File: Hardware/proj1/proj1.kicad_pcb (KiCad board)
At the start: 2 copper layers, 0 parts

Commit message: LED project layout
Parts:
- added D1: Red, layout:LED_0603_Symbol_on_F.SilkS, F.Cu at (119.5, 111.0)
- added J1: Conn_01x02, Connector_Molex:Molex_KK-254_AE-6410-02A_1x02_P2.54mm_Vertical, F.Cu at (103.0, 115.5)
- added R1: 105, Resistor_SMD:R_0603_1608Metric_Pad0.98x0.95mm_HandSolder, F.Cu at (119.6, 107.0)
- added SW1: SW_Push, Button_Switch_THT:SW_PUSH_6mm, F.Cu at (109.2, 107.8)
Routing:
- net +3V3: track 0.00 -> 21.1 mm
- net GND: track 0.00 -> 16.7 mm
- net Net-(D1-A): track 0.00 -> 9.97 mm
- net Net-(R1-Pad1): track 0.00 -> 9.74 mm
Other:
- board outline added: 25 x 20 mm

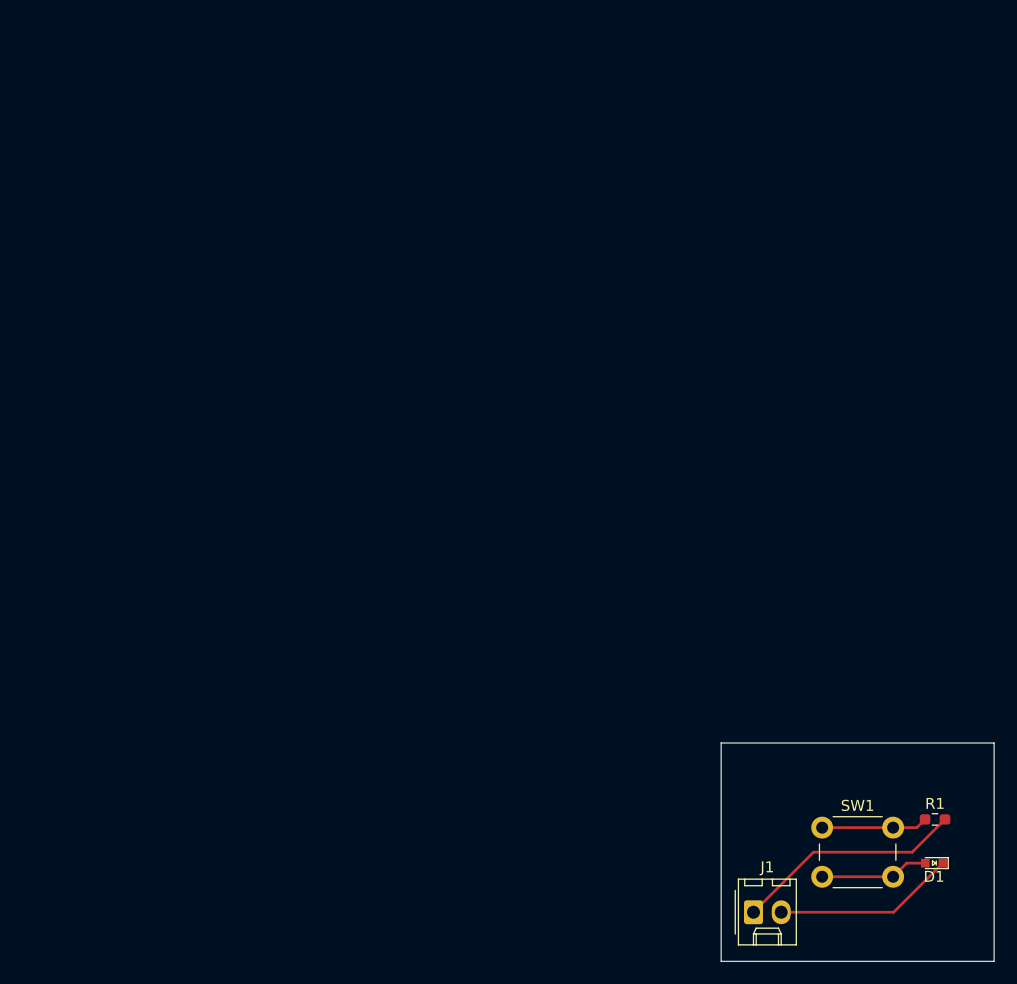
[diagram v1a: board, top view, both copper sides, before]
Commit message: Redo LED board PCB
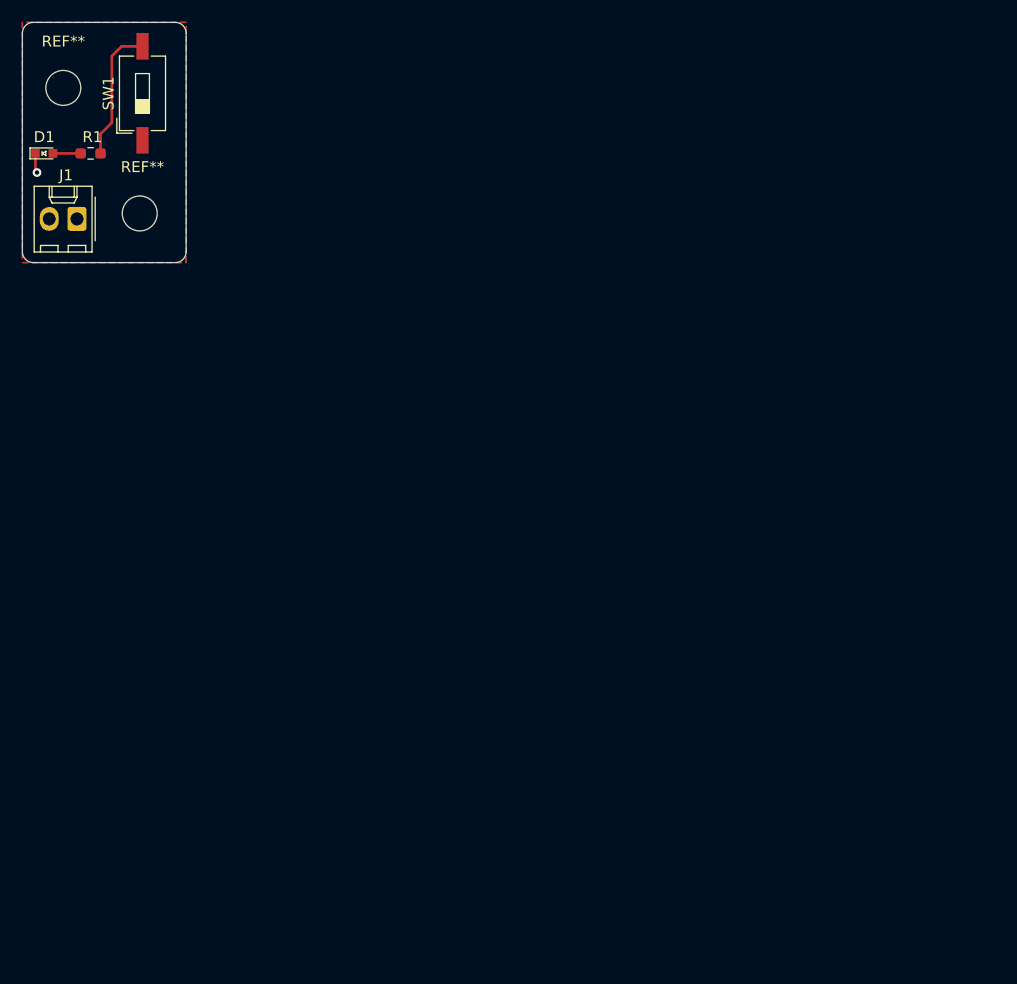
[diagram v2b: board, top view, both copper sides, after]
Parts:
- added REF**: MountingHole_3.2mm_M3, MountingHole:MountingHole_3.2mm_M3, F.Cu at (39.8, 40.0)
- added REF**: MountingHole_3.2mm_M3, MountingHole:MountingHole_3.2mm_M3, F.Cu at (46.8, 51.5)
- SW1: footprint Button_Switch_THT:SW_PUSH_6mm -> Button_Switch_SMD:SW_DIP_SPSTx01_Slide_6.7x4.1mm_W8.61mm_P2.54mm_LowProfile
- moved D1 104.2 mm to (38.0, 46.0), turned to 0 degrees
- moved R1 98.5 mm to (42.2, 46.0), turned to 180 degrees
- moved SW1 91.6 mm to (47.0, 40.5), turned to 90 degrees
- moved J1 88.7 mm to (41.0, 52.0), turned to 180 degrees
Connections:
- J1 pad 1: +3V3 -> GND
- J1 pad 2: GND -> +3V3
- R1 pad 2: +3V3 -> Net-(D1-A)
- SW1 pad 1: Net-(R1-Pad1) -> +3V3
- SW1 pad 2: Net-(D1-A) -> Net-(R1-Pad1)
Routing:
- net +3V3: track 21.1 -> 0.00 mm
- net GND: track 16.7 -> 1.81 mm, vias 0 -> 1
- net Net-(D1-A): track 9.97 -> 2.54 mm
- net Net-(R1-Pad1): track 9.74 -> 12.5 mm
- added copper zone on F.Cu, net +3V3
- added copper zone on B.Cu, net GND
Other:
- board size 25 x 20 mm -> 15 x 22 mm
